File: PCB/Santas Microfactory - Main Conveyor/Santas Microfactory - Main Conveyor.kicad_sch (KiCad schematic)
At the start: 179 parts, among them J1 Bus_PCI_Express_x16, J2 Conn_01x10_Pin, J3 Conn_01x10_Pin, Q1 NPN, Q10 NPN, Q11 NPN, Q12 NPN, Q13 NPN, Q14 NPN, Q15 NPN, Q16 NPN, Q17 NPN, Q18 NPN, Q19 NPN, Q2 NPN, Q20 NPN, Q21 NPN, Q22 NPN, Q23 NPN, Q24 NPN, Q3 NPN, Q4 NPN, Q5 NPN, Q6 NPN, Q7 NPN, Q8 NPN, Q9 NPN

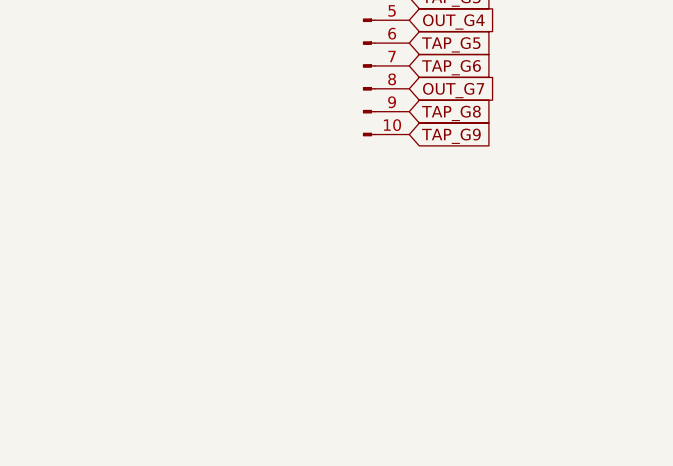
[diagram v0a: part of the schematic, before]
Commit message: Update Input Output Board
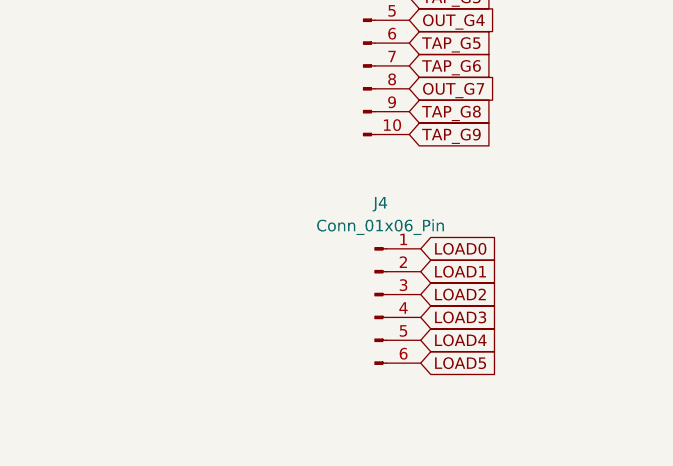
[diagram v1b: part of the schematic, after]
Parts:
- added J4: Conn_01x06_Pin, Connector_PinHeader_2.54mm:PinHeader_1x06_P2.54mm_Horizontal, symbol Connector:Conn_01x06_Pin
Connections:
- net LOAD0: now also J4.1 (Pin_1)
- net LOAD1: now also J4.2 (Pin_2)
- net LOAD2: now also J4.3 (Pin_3)
- net LOAD3: now also J4.4 (Pin_4)
- net LOAD4: now also J4.5 (Pin_5)
- net LOAD5: now also J4.6 (Pin_6)
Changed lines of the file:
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@@
 		)
 	)
+	(global_label "LOAD4"
+		(shape input)
+		(at 758.19 308.61 0)
+		(fields_autoplaced yes)
+		(effects
+			(font
+				(size 1.27 1.27)
+			)
+			(justify left)
+		)
+		(property "Intersheetrefs" "${INTERSHEET_REFS}"
+			(at 767.1019 308.61 0)
+			(effects
+				(font
+					(size 1.27 1.27)
+				)
+				(justify left)
+				(hide yes)
+			)
+		)
+	)
 	(global_label "NLOAD4"
 		(shape input)
@@
 		)
 	)
+	(global_label "LOAD5"
+		(shape input)
+		(at 758.19 311.15 0)
+		(fields_autoplaced yes)
+		(effects
+			(font
+				(size 1.27 1.27)
+			)
+			(justify left)
+		)
+		(property "Intersheetrefs" "${INTERSHEET_REFS}"
+			(at 767.1019 311.15 0)
+			(effects
+				(font
+					(size 1.27 1.27)
+				)
+				(justify left)
+				(hide yes)
+			)
+		)
+	)
 	(global_label "REQ3"
 		(shape input)
@@
 		)
 	)
+	(global_label "LOAD1"
+		(shape input)
+		(at 758.19 300.99 0)
+		(fields_autoplaced yes)
+		(effects
+			(font
+				(size 1.27 1.27)
+			)
+			(justify left)
+		)
+		(property "Intersheetrefs" "${INTERSHEET_REFS}"
+			(at 767.1019 300.99 0)
+			(effects
+				(font
+					(size 1.27 1.27)
+				)
+				(justify left)
+				(hide yes)
+			)
+		)
+	)
 	(global_label "INPUT4"
 		(shape input)
@@
 		)
 	)
+	(global_label "LOAD2"
+		(shape input)
+		(at 758.19 303.53 0)
+		(fields_autoplaced yes)
+		(effects
+			(font
+				(size 1.27 1.27)
+			)
+			(justify left)
+		)
+		(property "Intersheetrefs" "${INTERSHEET_REFS}"
+			(at 767.1019 303.53 0)
+			(effects
+				(font
+					(size 1.27 1.27)
+				)
+				(justify left)
+				(hide yes)
+			)
+		)
+	)
 	(global_label "NRESET"
 		(shape input)
@@
 		)
 	)
+	(global_label "LOAD3"
+		(shape input)
+		(at 758.19 306.07 0)
+		(fields_autoplaced yes)
+		(effects
+			(font
+				(size 1.27 1.27)
+			)
+			(justify left)
+		)
+		(property "Intersheetrefs" "${INTERSHEET_REFS}"
+			(at 767.1019 306.07 0)
+			(effects
+				(font
+					(size 1.27 1.27)
+				)
+				(justify left)
+				(hide yes)
+			)
+		)
+	)
 	(global_label "NHALT"
 		(shape input)
@@
 		)
 	)
+	(global_label "LOAD0"
+		(shape input)
+		(at 758.19 298.45 0)
+		(fields_autoplaced yes)
+		(effects
+			(font
+				(size 1.27 1.27)
+			)
+			(justify left)
+		)
+		(property "Intersheetrefs" "${INTERSHEET_REFS}"
+			(at 767.1019 298.45 0)
+			(effects
+				(font
+					(size 1.27 1.27)
+				)
+				(justify left)
+				(hide yes)
+			)
+		)
+	)
 	(global_label "TAP_G5"
 		(shape input)
@@
 					(unit 1)
 				)
+			)
+		)
+	)
+	(symbol
+		(lib_id "Connector:Conn_01x06_Pin")
+		(at 753.11 303.53 0)
+		(unit 1)
+		(exclude_from_sim no)
+		(in_bom yes)
+		(on_board yes)
+		(dnp no)
+		(fields_autoplaced yes)
+		(property "Reference" "J4"
+			(at 753.745 293.37 0)
+			(effects
+				(font
+					(size 1.27 1.27)
+				)
+			)
+		)
+		(property "Value" "Conn_01x06_Pin"
+			(at 753.745 295.91 0)
+			(effects
+				(font
+					(size 1.27 1.27)
+				)
+			)
+		)
+		(property "Footprint" "Connector_PinHeader_2.54mm:PinHeader_1x06_P2.54mm_Horizontal"
+			(at 753.11 303.53 0)
+			(effects
+				(font
+					(size 1.27 1.27)
+				)
+				(hide yes)
+			)
+		)
+		(property "Datasheet" "~"
+			(at 753.11 303.53 0)
+			(effects
+				(font
+					(size 1.27 1.27)
+				)
+				(hide yes)
+			)
+		)
+		(property "Description" "Generic connector, single row, 01x06, script generated"
+			(at 753.11 303.53 0)
+			(effects
+				(font
+					(size 1.27 1.27)
+				)
+				(hide yes)
+			)
+		)
+		(pin "4"
+		)
+		(pin "1"
+		)
+		(pin "2"
+		)
+		(pin "3"
+		)
+		(pin "6"
+		)
+		(pin "5"
+		)
+		(instances
+			(project ""
+				(path "/91c9ff6b-da3f-43a7-8acc-896df24b361f"
+					(reference "J4")
+					(unit 1)
+				)
